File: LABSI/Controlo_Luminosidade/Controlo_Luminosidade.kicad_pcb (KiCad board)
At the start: 2 copper layers, 60 x 80 mm, 41 parts, among them J1 5V/4A, J10 Touch Button, J11 Touch Button, J12 Touch Button, J2 Barrel_Jack_Switch, J3 Conn_01x05_Pin, J4 Conn_01x04_Pin, J5 Conn_01x04_Pin, J6 AVR-ISP-6, J7 Conn_01x03_Pin, J8 Conn_01x03_Pin, J9 Conn_01x05_Pin, Q1 IRLZ24, U1 ATmega328-P, U4 I2C_4PIN, Y1 16M

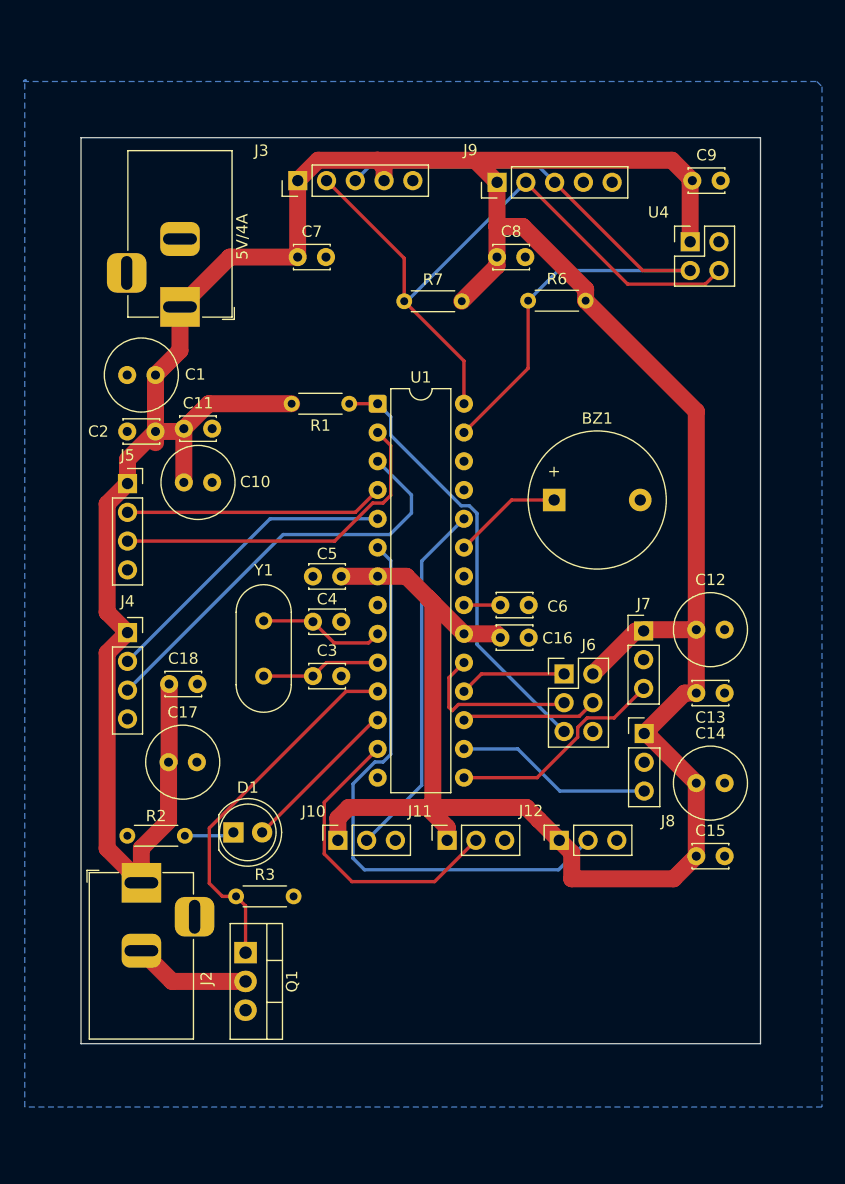
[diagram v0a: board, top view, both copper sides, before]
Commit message: pcb finalizado, gee«rbers gerados, falta desenvolver o que falta no ultimo commit
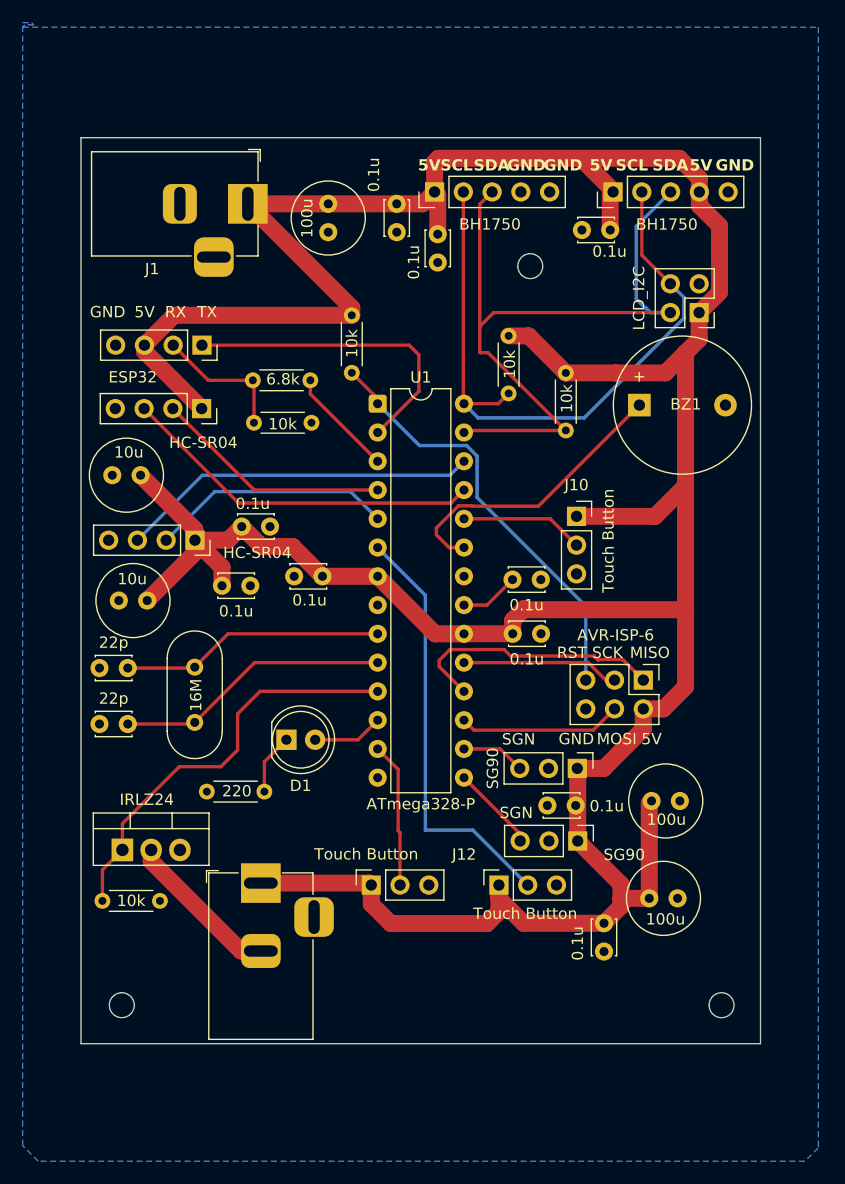
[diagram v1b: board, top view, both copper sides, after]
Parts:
- removed C9: 0.1u, Capacitor_THT:C_Disc_D3.0mm_W2.0mm_P2.50mm
- added J13: ESP32, Connector_PinSocket_2.54mm:PinSocket_1x04_P2.54mm_Vertical, F.Cu at (135.8, 68.2)
- added R8: 6.8k, Resistor_THT:R_Axial_DIN0204_L3.6mm_D1.6mm_P5.08mm_Horizontal, F.Cu at (145.3, 71.3)
- added R9: 10k, Resistor_THT:R_Axial_DIN0204_L3.6mm_D1.6mm_P5.08mm_Horizontal, F.Cu at (140.3, 75.0)
- added REF**: MountingHole_2.2mm_M2, MountingHole:MountingHole_2.2mm_M2, F.Cu at (164.7, 61.2)
- added REF**: MountingHole_2.2mm_M2, MountingHole:MountingHole_2.2mm_M2, F.Cu at (181.6, 126.5)
- added REF**: MountingHole_2.2mm_M2, MountingHole:MountingHole_2.2mm_M2, F.Cu at (128.7, 126.5)
- J1: value 5V/4A -> Barrel_Jack_Switch
- J3, J9: value Conn_01x05_Pin -> BH1750
- J4, J5: value Conn_01x04_Pin -> HC-SR04
- J7, J8: value Conn_01x03_Pin -> SG90
- U4: value I2C_4PIN -> LCD_I2C; footprint Connector_PinHeader_2.54mm:PinHeader_2x02_P2.54mm_Vertical -> Connector_PinSocket_2.54mm:PinSocket_2x02_P2.54mm_Vertical
- moved J10 35.5 mm to (168.8, 83.3), turned to 0 degrees
- moved C2 29.3 mm to (152.9, 55.7), turned to -90 degrees
- moved J3 27.9 mm to (172.1, 54.6)
- moved C7 27.7 mm to (171.8, 58.0), turned to 180 degrees
- moved C12 24.1 mm to (175.2, 117.0)
- moved C13 21.9 mm to (171.2, 119.2), turned to -90 degrees
- moved C1 21.5 mm to (146.9, 55.7), turned to -90 degrees
- moved J7 19.4 mm to (168.9, 112.0), turned to -90 degrees
- moved C3 16.9 mm to (129.2, 101.6), turned to 180 degrees
- moved C4 16.9 mm to (129.2, 96.7), turned to 180 degrees
- moved C17 14.4 mm to (130.9, 90.7), turned to 180 degrees
- moved Q1 14.2 mm to (128.7, 112.8), turned to 0 degrees
- moved R7 12.3 mm to (162.8, 72.4), turned to 90 degrees
- moved R6 11.9 mm to (167.9, 75.7), turned to 90 degrees
- moved R3 11.8 mm to (127.0, 117.2)
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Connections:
- net /PD5/GATE renamed /PB3/GATE
- U1 pad 2: /TRIG -> /RX_ATMEGA
- U1 pad 25: unconnected-(U1-PC2-Pad25) -> /TRIG
- U1 pad 26: unconnected-(U1-PC3-Pad26) -> /TRIG2
- U1 pad 3: /TRIG2 -> /TX_ATMEGA
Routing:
- net /RX_ATMEGA: track 0.00 -> 27.9 mm
- net Net-(J10-Pin_2): track 32.0 -> 10.9 mm
- net /BUZZER: track 9.70 -> 26.0 mm
- net /PD7/SW2: track 27.1 -> 12.8 mm
- net /PD4/SW1: track 52.0 -> 37.7 mm
- net /MISO: track 9.48 -> 23.3 mm
- net /XTAL2: track 10.6 -> 24.3 mm
- net /XTAL1: track 11.2 -> 23.3 mm
- net /RX_ESP-32: track 0.00 -> 12.1 mm
- net /SERVO1: track 19.6 -> 7.65 mm
- net /SERVO2: track 17.5 -> 5.64 mm
- net /TX_ATMEGA: track 0.00 -> 9.61 mm
- net +5V: track 328.1 -> 319.0 mm
- net Net-(D1-A): track 14.3 -> 6.24 mm
- net /ECHO2: track 27.3 -> 21.4 mm
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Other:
- copper layers 2 -> 4
- board text added: "5V"
- board text added: "GND"
- board text added: "MISO"
- board text added: "MOSI"
- board text added: "RST"
- board text added: "RX"
- board text added: "SCK"
- board text added: "SCL"
- board text added: "SDA"
- board text added: "SGN"
- board text added: "TX"
